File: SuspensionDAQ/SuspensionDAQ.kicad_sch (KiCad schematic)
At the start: 14 parts, among them U1 Teensy4.1, U2 module_mpu6050, U5 TPS613222ADBV

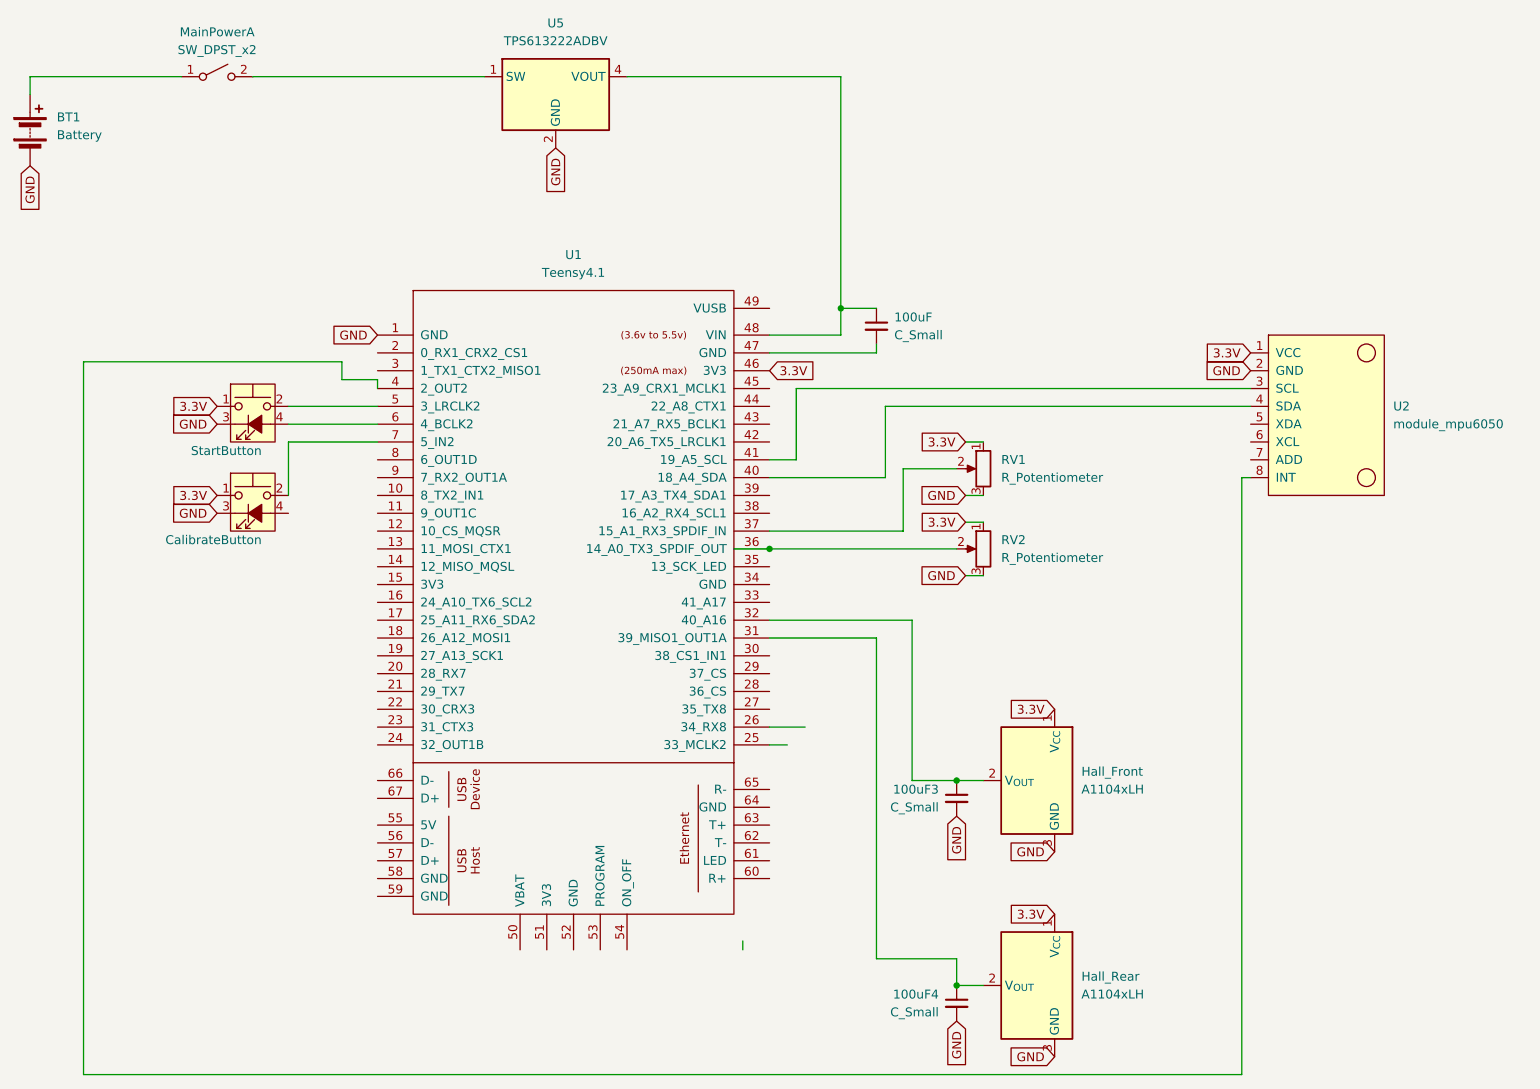
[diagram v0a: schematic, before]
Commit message: WIP
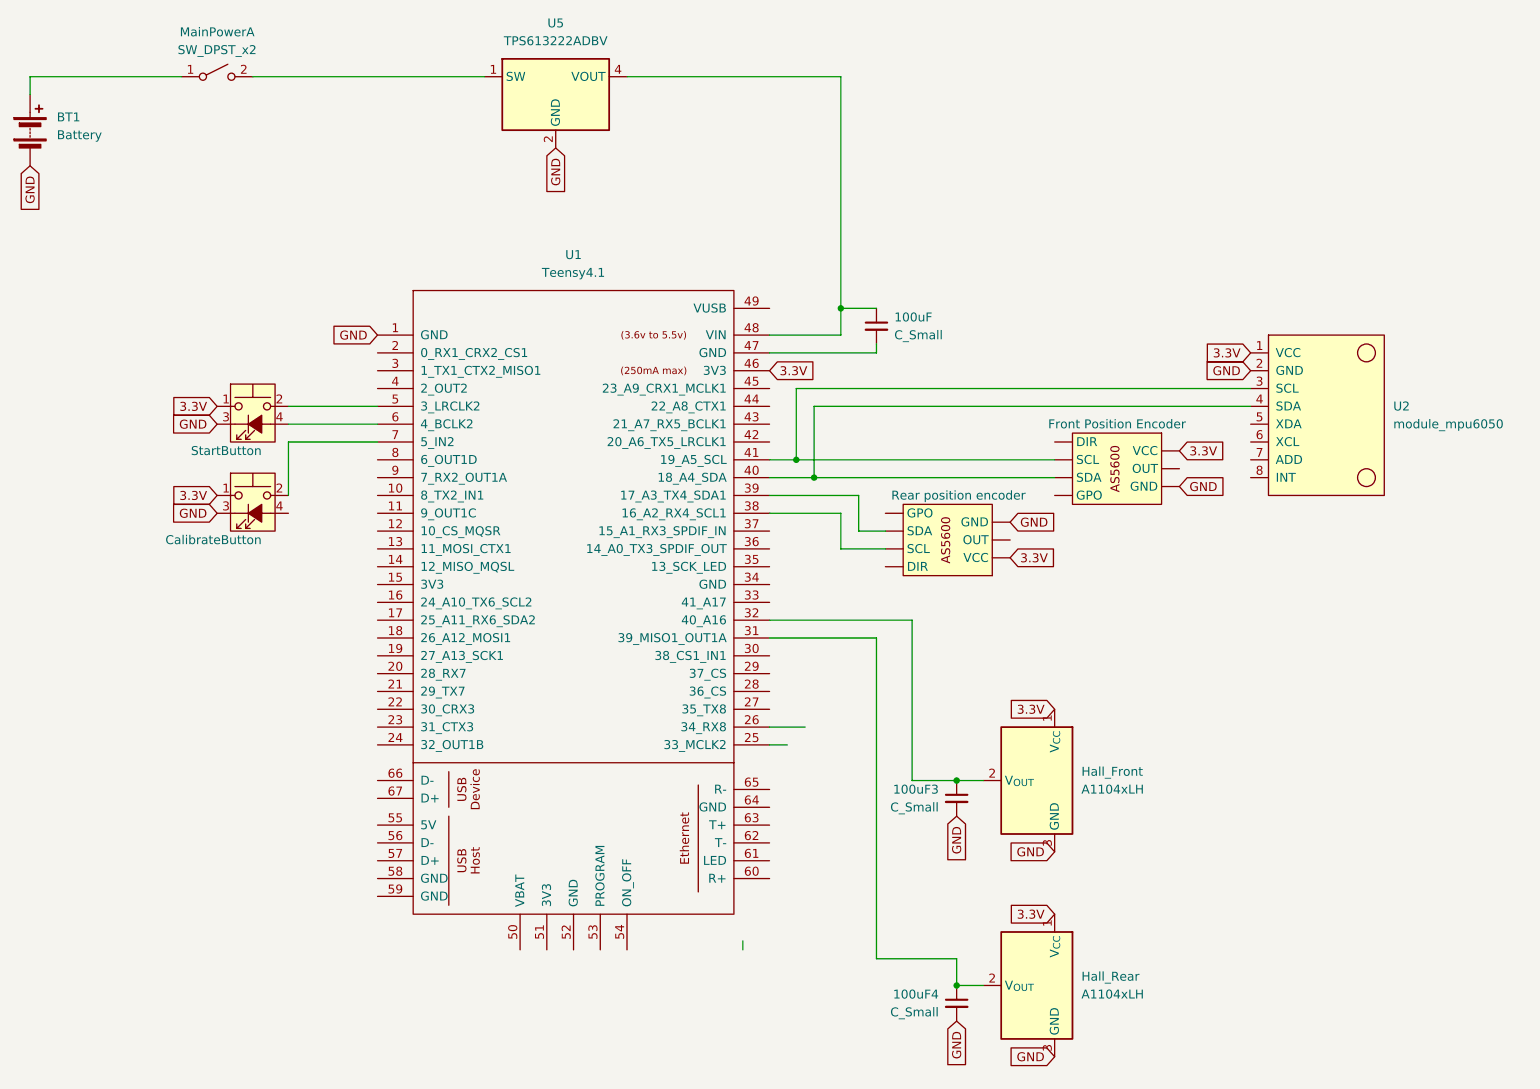
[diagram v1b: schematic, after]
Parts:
- removed RV1, RV2: R_Potentiometer, symbol Device:R_Potentiometer
- added U3: Front Position Encoder, symbol AS5600:AS5600
- added U4: Rear position encoder, symbol AS5600:AS5600
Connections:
- net 3.3V: now also U3. (GPO), U4. (GPO)
- net GND: now also U3. (GPO), U4. (GPO)
- net at U1.38 (16_A2_RX4_SCL1): now also U4. (GPO)
- net at U1.39 (17_A3_TX4_SDA1): now also U4. (GPO)
- net at U1.4 (2_OUT2): no longer U2.8 (INT)
- net at U1.40 (18_A4_SDA), U2.4 (SDA): now also U3. (GPO)
- net at U1.41 (19_A5_SCL), U2.3 (SCL): now also U3. (GPO)
